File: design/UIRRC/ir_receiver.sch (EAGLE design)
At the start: 3 parts, among them IC1 TSOP38438

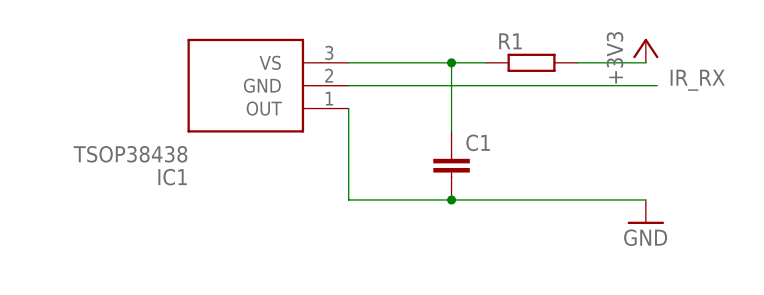
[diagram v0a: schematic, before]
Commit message: Fixes #3
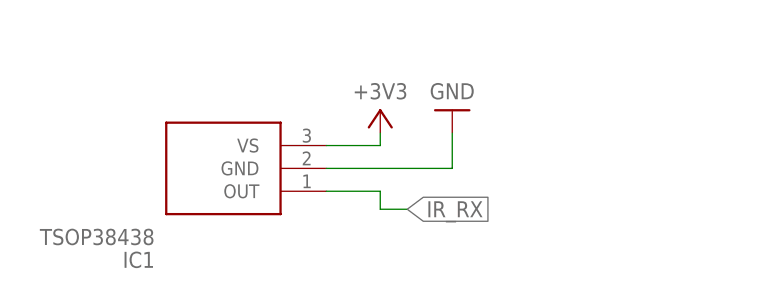
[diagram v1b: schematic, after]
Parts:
- removed C1: (no value), rcl:C-EUC3225
- removed R1: (no value), rcl:R-EU_R1206
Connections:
- removed net N$1: C1.1, IC1.VS, R1.1
- net +3V3: now also IC1.VS; no longer R1.2
- net GND: now also IC1.GND; no longer C1.2, IC1.OUT
- net IR_RX: now also IC1.OUT; no longer IC1.GND
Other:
- moved on the sheet: IC1
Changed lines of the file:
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@@
 <setting verticaltext="up"/>
 </settings>
-<grid distance="0.1" unitdist="inch" unit="inch" style="lines" multiple="1" display="no" altdistance="0.01" altunitdist="inch" altunit="inch"/>
+<grid distance="1" unitdist="mm" unit="mm" style="lines" multiple="1" display="yes" altdistance="1" altunitdist="mm" altunit="mm"/>
 <layers>
 <layer number="1" name="Top" color="4" fill="1" visible="no" active="no"/>
@@
 </classes>
 <parts>
-<part name="FRAME1" library="frames" library_urn="urn:adsk.eagle:library:229" deviceset="DINA4_L" device=""/>
+<part name="FRAME1" library="frames" library_urn="urn:adsk.eagle:library:229" deviceset="DINA5_L" device=""/>
 <part name="IC1" library="TSOP38438" deviceset="TSOP38438" device=""/>
 <part name="+3V1" library="supply1" library_urn="urn:adsk.eagle:library:371" deviceset="+3V3" device=""/>
 <part name="GND1" library="supply1" library_urn="urn:adsk.eagle:library:371" deviceset="GND" device=""/>
-<part name="C1" library="rcl" library_urn="urn:adsk.eagle:library:334" deviceset="C-EU" device="C3225" package3d_urn="urn:adsk.eagle:package:23655/2"/>
-<part name="R1" library="rcl" library_urn="urn:adsk.eagle:library:334" deviceset="R-EU_" device="R1206" package3d_urn="urn:adsk.eagle:package:23540/2"/>
 </parts>
 <sheets>
@@
 </plain>
 <instances>
-<instance part="FRAME1" gate="G$1" x="16.51" y="-5.08" smashed="yes"/>
-<instance part="FRAME1" gate="G$2" x="179.07" y="-5.08" smashed="yes">
-<attribute name="LAST_DATE_TIME" x="191.77" y="-3.81" size="2.54" layer="94"/>
-<attribute name="SHEET" x="265.43" y="-3.81" size="2.54" layer="94"/>
-<attribute name="DRAWING_NAME" x="196.85" y="13.97" size="2.54" layer="94"/>
+<instance part="FRAME1" gate="G$1" x="27.94" y="48.26" smashed="yes">
+<attribute name="DRAWING_NAME" x="168.91" y="63.5" size="2.54" layer="94"/>
+<attribute name="LAST_DATE_TIME" x="168.91" y="58.42" size="2.286" layer="94"/>
+<attribute name="SHEET" x="182.245" y="53.34" size="2.54" layer="94"/>
 </instance>
-<instance part="IC1" gate="G$1" x="110.49" y="123.19" smashed="yes" rot="R180">
-<attribute name="NAME" x="92.71" y="115.57" size="1.778" layer="95" rot="R180" align="center-left"/>
-<attribute name="VALUE" x="92.71" y="118.11" size="1.778" layer="96" rot="R180" align="center-left"/>
+<instance part="IC1" gate="G$1" x="108" y="114" smashed="yes" rot="R180">
+<attribute name="NAME" x="88.95" y="106.38" size="1.778" layer="95" rot="R180" align="center-left"/>
+<attribute name="VALUE" x="88.95" y="108.92" size="1.778" layer="96" rot="R180" align="center-left"/>
 </instance>
-<instance part="+3V1" gate="G$1" x="143.51" y="130.81" smashed="yes">
-<attribute name="VALUE" x="140.97" y="125.73" size="1.778" layer="96" rot="R90"/>
+<instance part="+3V1" gate="G$1" x="114" y="123" smashed="yes">
+<attribute name="VALUE" x="114" y="126" size="1.778" layer="96" rot="R180" align="bottom-center"/>
 </instance>
-<instance part="GND1" gate="1" x="143.51" y="110.49" smashed="yes">
-<attribute name="VALUE" x="140.97" y="107.95" size="1.778" layer="96"/>
-</instance>
-<instance part="C1" gate="G$1" x="121.92" y="118.11" smashed="yes">
-<attribute name="NAME" x="123.444" y="118.491" size="1.778" layer="95"/>
-<attribute name="VALUE" x="123.444" y="113.411" size="1.778" layer="96"/>
-</instance>
-<instance part="R1" gate="G$1" x="130.81" y="128.27" smashed="yes">
-<attribute name="NAME" x="127" y="129.7686" size="1.778" layer="95"/>
-<attribute name="VALUE" x="127" y="124.968" size="1.778" layer="96"/>
+<instance part="GND1" gate="1" x="122" y="123" smashed="yes" rot="R180">
+<attribute name="VALUE" x="122" y="126" size="1.778" layer="96" rot="R180" align="bottom-center"/>
 </instance>
 </instances>
@@
 </busses>
 <nets>
-<net name="N$1" class="0">
+<net name="+3V3" class="0">
 <segment>
 <pinref part="IC1" gate="G$1" pin="VS"/>
-<pinref part="R1" gate="G$1" pin="1"/>
-<wire x1="110.49" y1="128.27" x2="121.92" y2="128.27" width="0.1524" layer="91"/>
-<pinref part="C1" gate="G$1" pin="1"/>
-<wire x1="121.92" y1="128.27" x2="125.73" y2="128.27" width="0.1524" layer="91"/>
-<wire x1="121.92" y1="120.65" x2="121.92" y2="128.27" width="0.1524" layer="91"/>
-<junction x="121.92" y="128.27"/>
-</segment>
-</net>
-<net name="+3V3" class="0">
-<segment>
-<pinref part="R1" gate="G$1" pin="2"/>
 <pinref part="+3V1" gate="G$1" pin="+3V3"/>
-<wire x1="135.89" y1="128.27" x2="143.51" y2="128.27" width="0.1524" layer="91"/>
+<wire x1="108" y1="119.08" x2="114" y2="119.08" width="0.1524" layer="91"/>
+<wire x1="114" y1="119.08" x2="114" y2="120.46" width="0.1524" layer="91"/>
 </segment>
 </net>
 <net name="GND" class="0">
 <segment>
-<pinref part="IC1" gate="G$1" pin="OUT"/>
+<pinref part="IC1" gate="G$1" pin="GND"/>
 <pinref part="GND1" gate="1" pin="GND"/>
-<wire x1="110.49" y1="123.19" x2="110.49" y2="113.03" width="0.1524" layer="91"/>
-<wire x1="110.49" y1="113.03" x2="121.92" y2="113.03" width="0.1524" layer="91"/>
-<pinref part="C1" gate="G$1" pin="2"/>
-<wire x1="121.92" y1="113.03" x2="143.51" y2="113.03" width="0.1524" layer="91"/>
-<junction x="121.92" y="113.03"/>
+<wire x1="108" y1="116.54" x2="122" y2="116.54" width="0.1524" layer="91"/>
+<wire x1="122" y1="116.54" x2="122" y2="120.46" width="0.1524" layer="91"/>
 </segment>
 </net>
 <net name="IR_RX" class="0">
 <segment>
-<pinref part="IC1" gate="G$1" pin="GND"/>
-<wire x1="110.49" y1="125.73" x2="144.78" y2="125.73" width="0.1524" layer="91"/>
-<label x="146.05" y="125.73" size="1.778" layer="95"/>
+<pinref part="IC1" gate="G$1" pin="OUT"/>
+<wire x1="108" y1="114" x2="114" y2="114" width="0.1524" layer="91"/>
+<wire x1="114" y1="114" x2="114" y2="112" width="0.1524" layer="91"/>
+<wire x1="114" y1="112" x2="117" y2="112" width="0.1524" layer="91"/>
+<label x="117" y="112" size="1.778" layer="95" xref="yes"/>
 </segment>
 </net>
@@
 will not be understood (or retained) with this version.
 </note>
-<note version="8.3" severity="warning">
-Since Version 8.3, EAGLE supports the association of 3D packages
-with devices in libraries, schematics, and board files. Those 3D
-packages will not be understood (or retained) with this version.
-</note>
-<note version="8.4" severity="warning">
-Since Version 8.4, EAGLE supports properties for SPICE simulation.
-Probes in schematics and SPICE mapping objects found in parts and library devices
-will not be understood with this version. Update EAGLE to the latest version
-for full support of SPICE simulation.
-</note>
 </compatibility>
